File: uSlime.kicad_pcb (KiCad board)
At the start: 2 copper layers, 26.1 x 21.7 mm, 22 parts, among them U2 AP2112K-3.3TRG1, U3 MCP73831T-2ACI/OT, U4 ESP32-C6FH4, U5 BNO085

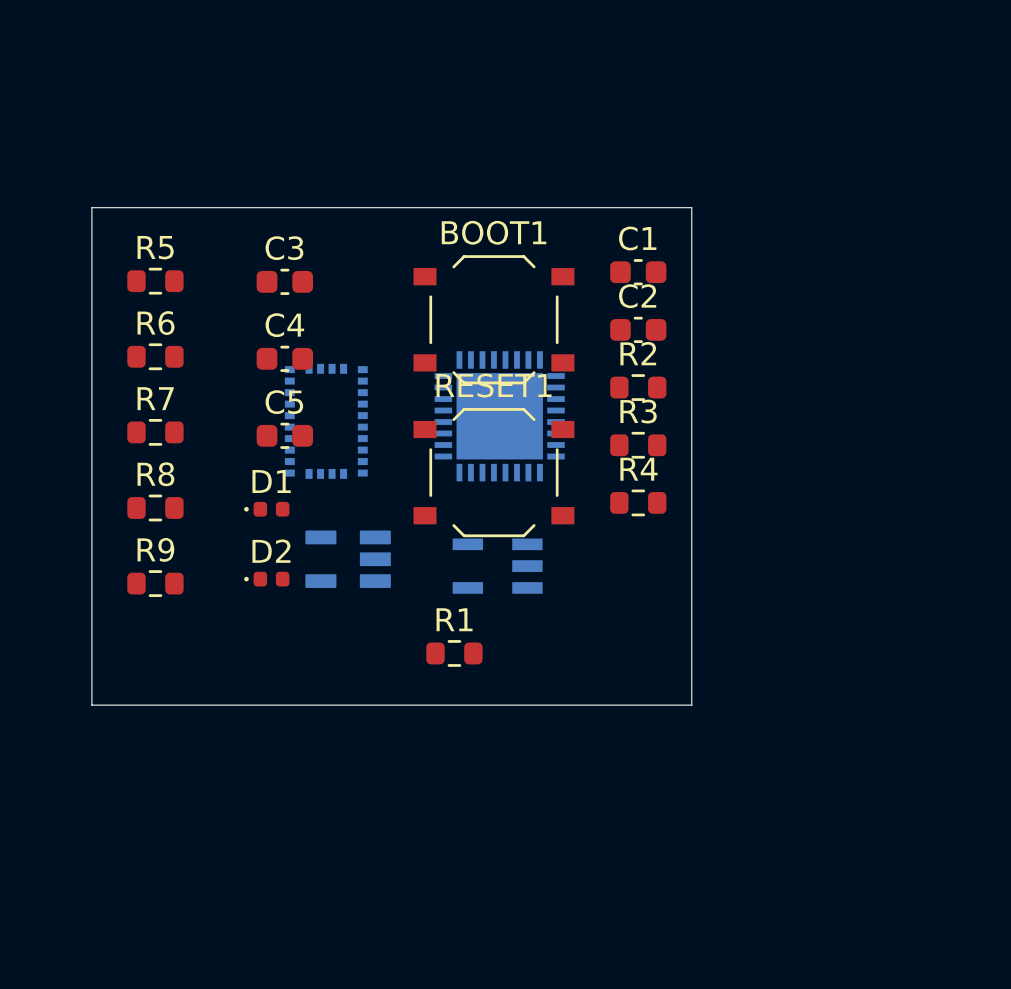
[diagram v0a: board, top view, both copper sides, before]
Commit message: Modify ESP32
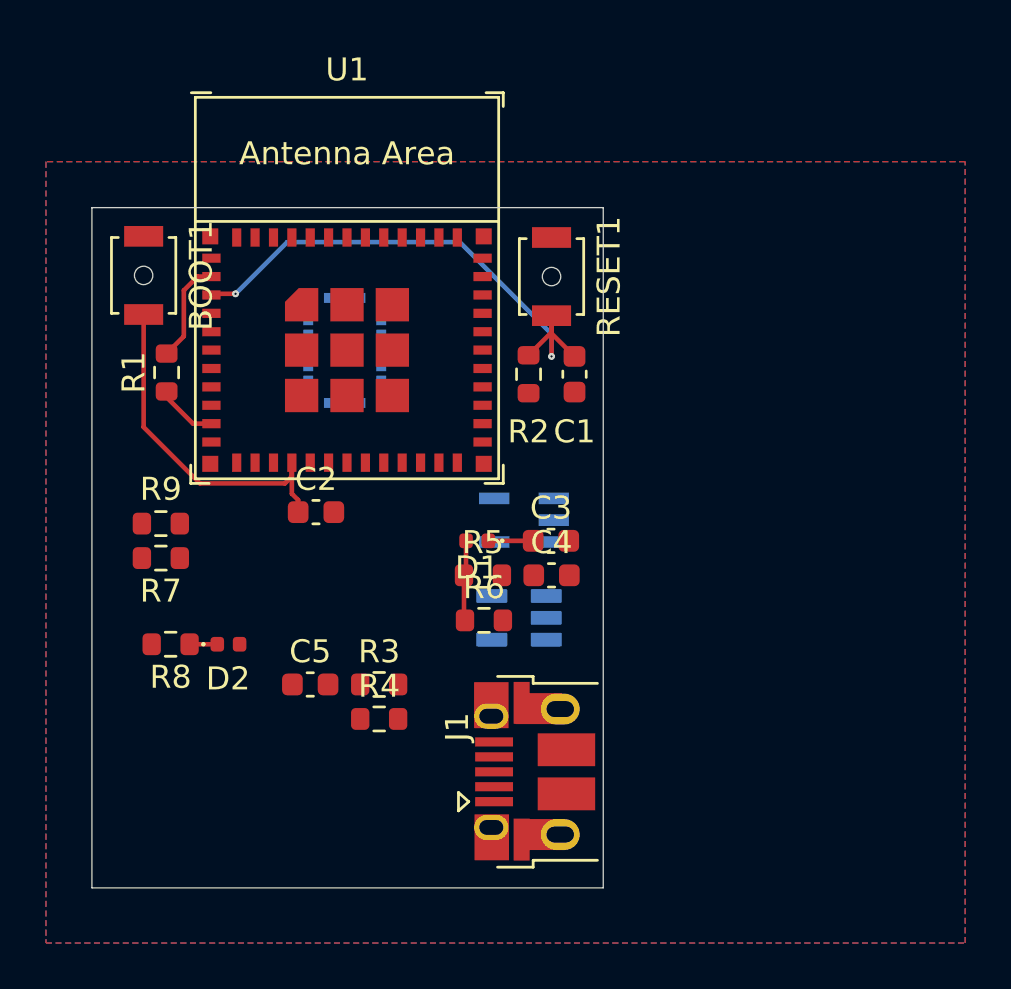
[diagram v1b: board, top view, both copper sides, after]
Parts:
- removed U4: ESP32-C6FH4, uSlime-libs:QFN32_ESP32_EXP
- added J1: USB_C_4-LAYER_PADS, Connector_USB:USB_Micro-B_Amphenol_10103594-0001LF_Horizontal, F.Cu at (119.9, 113.9)
- added U1: ESP32-C6-WROOM-1-NARROW, PCM_Espressif:ESP32-C6-MINI-1, F.Cu at (111.8, 92.8)
- BOOT1, RESET1: value MOMENTARY-SWITCH-SPST-SMD-4.6X2.8MM -> SW_Push; footprint Button_Switch_SMD:SW_Push_1P1T_XKB_TS-1187A -> Button_Switch_SMD:SW_SPST_B3U-1000P-B
- moved R5 19.2 mm to (117.7, 105.3)
- moved R6 18.3 mm to (117.7, 107.3)
- moved R1 17.5 mm to (103.9, 96.5), turned to 90 degrees
- moved C3 16.2 mm to (120.6, 103.8)
- moved C2 16.1 mm to (110.4, 102.6)
- moved BOOT1 15.4 mm to (102.9, 92.3), turned to -90 degrees
- moved R3 15.3 mm to (113.2, 110.1)
- moved C4 14.9 mm to (120.7, 105.3)
- moved R4 14.7 mm to (113.2, 111.6)
- moved C5 10.9 mm to (110.2, 110.1)
- moved D1 9.06 mm to (117.4, 103.8), turned to 180 degrees
- moved RESET1 8.89 mm to (120.7, 92.3), turned to -90 degrees
- moved U2 7.86 mm to (119.2, 107.2)
- moved R8 5.97 mm to (104.1, 108.3), turned to 180 degrees
- moved R7 5.48 mm to (103.7, 104.6), turned to 180 degrees
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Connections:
- BOOT1 pad 2: GND -> /ESP32-C6FH4/IO9/BOOT
- C5 pad 2: Net-(U3-VBAT) -> unconnected-(C5-Pad2)
- D2 pad 2: Net-(D2-A) -> unconnected-(D2-A-Pad2)
- R1 pad 2: 3.3V -> +3.3V
- R3 pad 2: Net-(J1-CC2) -> unconnected-(R3-Pad2)
- R4 pad 2: Net-(J1-CC1) -> unconnected-(R4-Pad2)
- R8 pad 2: Net-(U3-STAT) -> unconnected-(R8-Pad2)
- RESET1 pad 2: GND -> /ESP32-C6FH4/ESP_EN
- U2 pad 3: Net-(D1-K) -> unconnected-(U2-EN-Pad3)
- U3 pad 1: Net-(U3-STAT) -> unconnected-(U3-STAT-Pad1)
- U3 pad 2: GND -> unconnected-(U3-VSS-Pad2)
- U3 pad 3: Net-(U3-VBAT) -> unconnected-(U3-VBAT-Pad3)
- U3 pad 4: Net-(D2-A) -> unconnected-(U3-VDD-Pad4)
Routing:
- net /ESP32-C6FH4/ESP_EN: track 0.00 -> 24.5 mm, vias 0 -> 2
- net /ESP32-C6FH4/IO9/BOOT: track 0.00 -> 15.4 mm
- net +3.3V: track 0.00 -> 4.51 mm
- net Net-(D1-A): track 0.00 -> 3.52 mm
- net /ESP32-C6FH4/IO8: track 0.00 -> 2.68 mm
- net Net-(D1-K): track 0.00 -> 1.95 mm
- net Net-(D2-K): track 0.00 -> 1.20 mm
- added copper zone on B.Cu, net GND
- added copper zone on F.Cu, net GND
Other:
- board size 26.1 x 21.7 mm -> 22.2 x 29.6 mm
